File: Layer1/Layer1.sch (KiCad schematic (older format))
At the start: 45 parts, among them IC1 74HCT4060D-Q100,11, J1 Conn_02x20_Odd_Even, J2 Conn_02x20_Odd_Even, J3 Conn_02x12_Odd_Even, J4 Barrel_Jack_MountingPin, SW1 SW_Push, SW2 SW_Push, SW3 SW_DIP_x01, U1 28C256, U10 7400, U11 NE555, U2 74LS193, U3 74461, U4 28C256, U5 74154, U6 74461, U7 28C256, U8 74HCT273, U9 28C256, X1 SG-8002DC

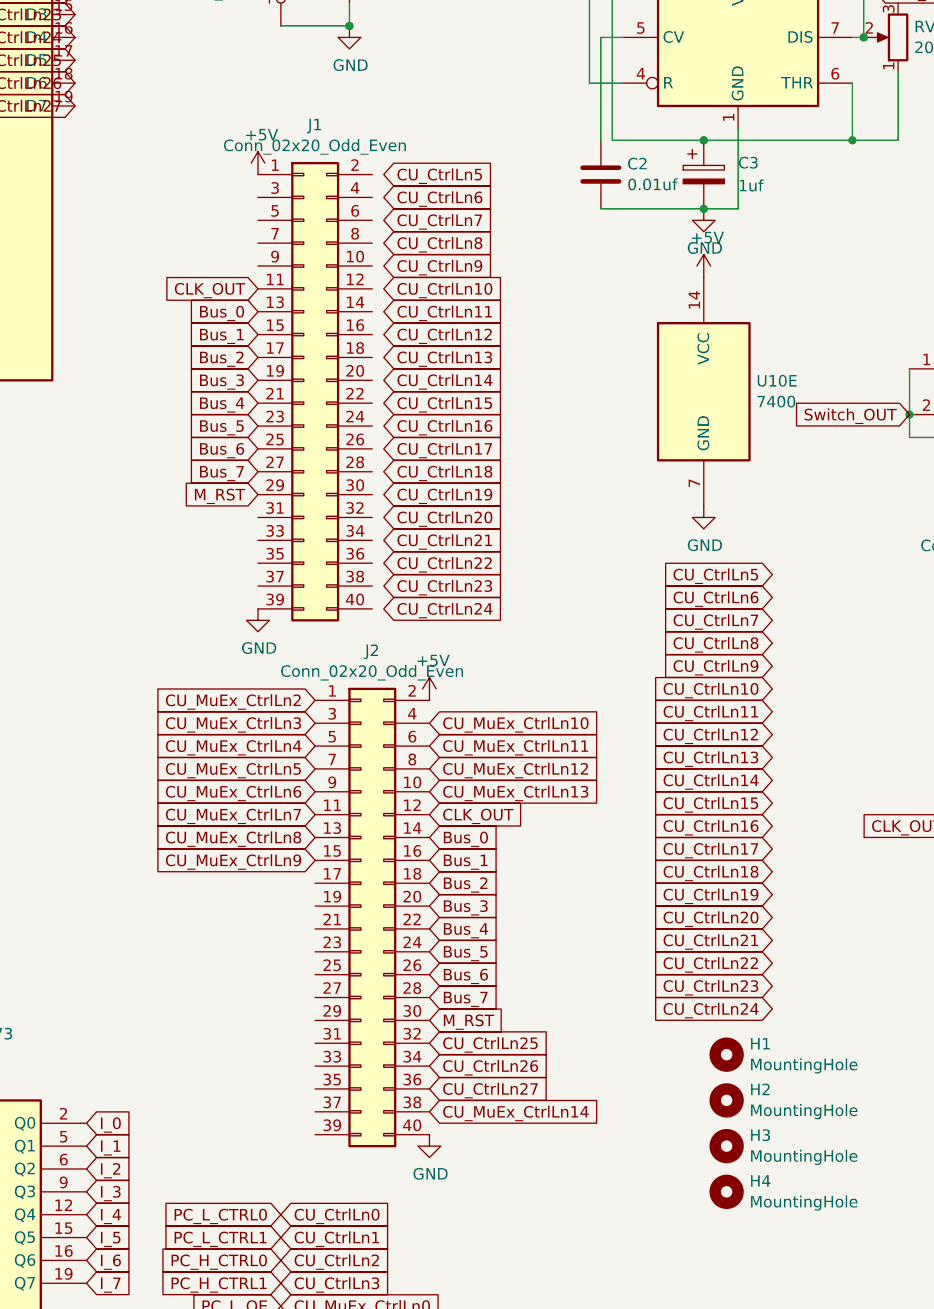
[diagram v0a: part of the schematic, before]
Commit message: Finished Layer1
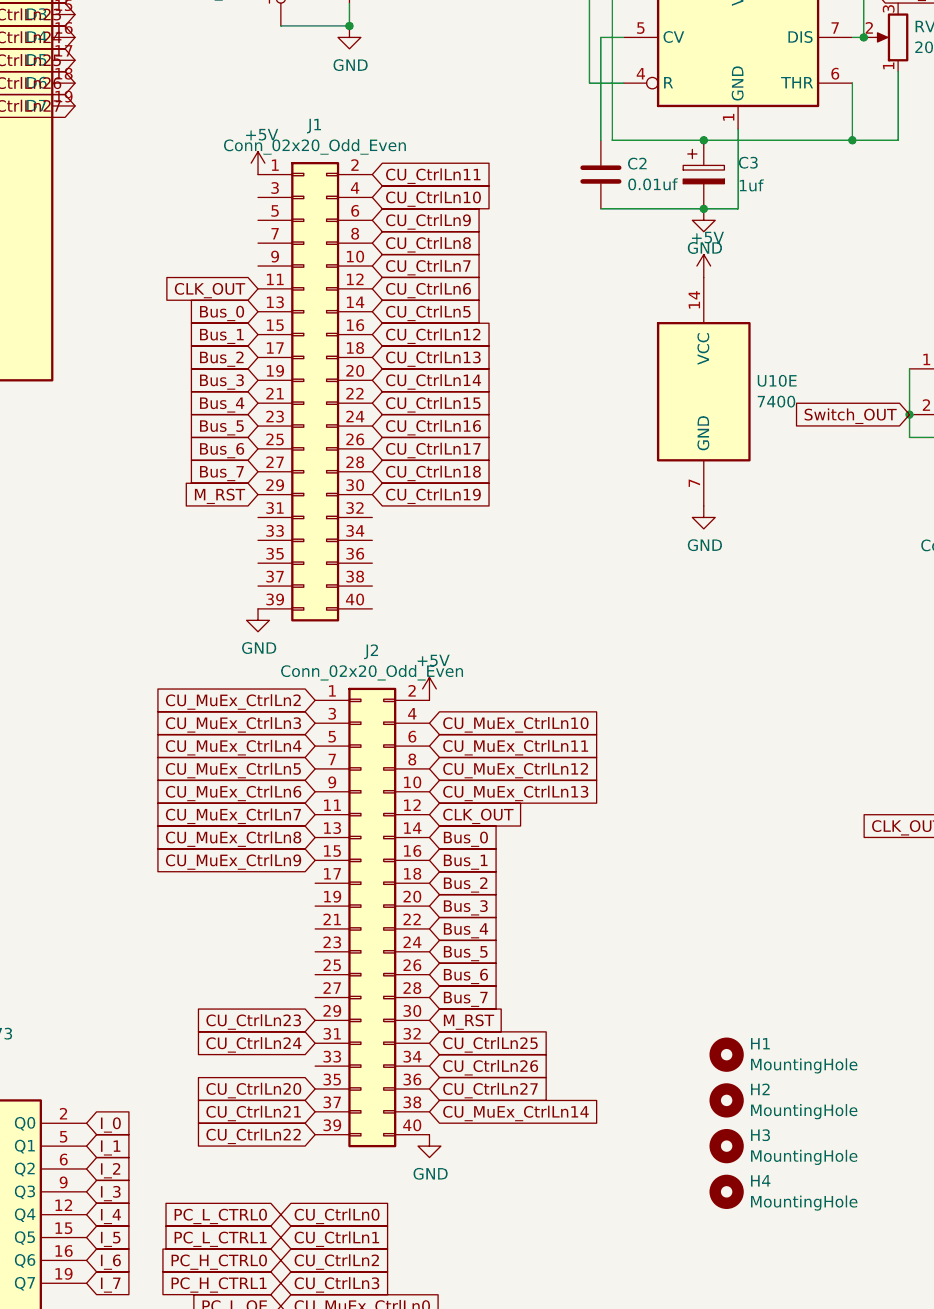
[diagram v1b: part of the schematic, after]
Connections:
- net CU_CtrlLn10: now also J1.4 (Pin_4)
- net CU_CtrlLn11: now also J1.2 (Pin_2)
- net CU_CtrlLn12: now also J1.16 (Pin_16)
- net CU_CtrlLn13: now also J1.18 (Pin_18)
- net CU_CtrlLn14: now also J1.20 (Pin_20)
- net CU_CtrlLn15: now also J1.22 (Pin_22)
- net CU_CtrlLn16: now also J1.24 (Pin_24)
- net CU_CtrlLn17: now also J1.26 (Pin_26)
- net CU_CtrlLn18: now also J1.28 (Pin_28)
- net CU_CtrlLn19: now also J1.30 (Pin_30)
- net CU_CtrlLn20: now also J2.35 (Pin_35)
- net CU_CtrlLn21: now also J2.37 (Pin_37)
- net CU_CtrlLn22: now also J2.39 (Pin_39)
- net CU_CtrlLn23: now also J2.29 (Pin_29)
- net CU_CtrlLn24: now also J2.31 (Pin_31)
- net CU_CtrlLn5: now also J1.14 (Pin_14)
- net CU_CtrlLn6: now also J1.12 (Pin_12)
- net CU_CtrlLn7: now also J1.10 (Pin_10)
- net CU_CtrlLn8: now also J1.8 (Pin_8)
- net CU_CtrlLn9: now also J1.6 (Pin_6)
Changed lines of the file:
@@
 Text GLabel 6600 6050 2    50   Input ~ 0
 CU_MuEx_CtrlLn14
-Text GLabel 6400 1950 2    50   Input ~ 0
-CU_CtrlLn5
-Text GLabel 6400 2050 2    50   Input ~ 0
-CU_CtrlLn6
-Text GLabel 6400 2150 2    50   Input ~ 0
-CU_CtrlLn7
-Text GLabel 6400 2250 2    50   Input ~ 0
-CU_CtrlLn8
-Text GLabel 6400 2350 2    50   Input ~ 0
-CU_CtrlLn9
-Text GLabel 6400 2450 2    50   Input ~ 0
-CU_CtrlLn10
-Text GLabel 6400 2550 2    50   Input ~ 0
-CU_CtrlLn11
-Text GLabel 6400 2650 2    50   Input ~ 0
+Text GLabel 6350 2650 2    50   Input ~ 0
 CU_CtrlLn12
-Text GLabel 6400 2750 2    50   Input ~ 0
+Text GLabel 6350 2750 2    50   Input ~ 0
 CU_CtrlLn13
-Text GLabel 6400 2850 2    50   Input ~ 0
+Text GLabel 6350 2850 2    50   Input ~ 0
 CU_CtrlLn14
-Text GLabel 6400 2950 2    50   Input ~ 0
+Text GLabel 6350 2950 2    50   Input ~ 0
 CU_CtrlLn15
-Text GLabel 6400 3050 2    50   Input ~ 0
+Text GLabel 6350 3050 2    50   Input ~ 0
 CU_CtrlLn16
-Text GLabel 6400 3150 2    50   Input ~ 0
+Text GLabel 6350 3150 2    50   Input ~ 0
 CU_CtrlLn17
-Text GLabel 6400 3250 2    50   Input ~ 0
+Text GLabel 6350 3250 2    50   Input ~ 0
 CU_CtrlLn18
-Text GLabel 6400 3350 2    50   Input ~ 0
+Text GLabel 6350 3350 2    50   Input ~ 0
 CU_CtrlLn19
-Text GLabel 6400 3450 2    50   Input ~ 0
-CU_CtrlLn20
-Text GLabel 6400 3550 2    50   Input ~ 0
-CU_CtrlLn21
-Text GLabel 6400 3650 2    50   Input ~ 0
-CU_CtrlLn22
-Text GLabel 6400 3750 2    50   Input ~ 0
-CU_CtrlLn23
-Text GLabel 6400 3850 2    50   Input ~ 0
-CU_CtrlLn24
 Text GLabel 6600 5750 2    50   Input ~ 0
 CU_CtrlLn25
@@
 Text GLabel 6600 5650 2    50   Input ~ 0
 M_RST
-Text GLabel 8100 3700 0    50   Input ~ 0
+Text GLabel 6100 5950 0    50   Input ~ 0
+CU_CtrlLn20
+Text GLabel 6100 6050 0    50   Input ~ 0
+CU_CtrlLn21
+Text GLabel 6100 6150 0    50   Input ~ 0
+CU_CtrlLn22
+Text GLabel 6100 5650 0    50   Input ~ 0
+CU_CtrlLn23
+Text GLabel 6100 5750 0    50   Input ~ 0
+CU_CtrlLn24
+Text GLabel 6350 1950 2    50   Input ~ 0
+CU_CtrlLn11
+Text GLabel 6350 2050 2    50   Input ~ 0
+CU_CtrlLn10
+Text GLabel 6350 2150 2    50   Input ~ 0
+CU_CtrlLn9
+Text GLabel 6350 2250 2    50   Input ~ 0
+CU_CtrlLn8
+Text GLabel 6350 2350 2    50   Input ~ 0
+CU_CtrlLn7
+Text GLabel 6350 2450 2    50   Input ~ 0
+CU_CtrlLn6
+Text GLabel 6350 2550 2    50   Input ~ 0
 CU_CtrlLn5
-Text GLabel 8100 3800 0    50   Input ~ 0
-CU_CtrlLn6
-Text GLabel 8100 3900 0    50   Input ~ 0
-CU_CtrlLn7
-Text GLabel 8100 4000 0    50   Input ~ 0
-CU_CtrlLn8
-Text GLabel 8100 4100 0    50   Input ~ 0
-CU_CtrlLn9
-Text GLabel 8100 4200 0    50   Input ~ 0
-CU_CtrlLn10
-Text GLabel 8100 4300 0    50   Input ~ 0
-CU_CtrlLn11
-Text GLabel 8100 4400 0    50   Input ~ 0
-CU_CtrlLn12
-Text GLabel 8100 4500 0    50   Input ~ 0
-CU_CtrlLn13
-Text GLabel 8100 4600 0    50   Input ~ 0
-CU_CtrlLn14
-Text GLabel 8100 4700 0    50   Input ~ 0
-CU_CtrlLn15
-Text GLabel 8100 4800 0    50   Input ~ 0
-CU_CtrlLn16
-Text GLabel 8100 4900 0    50   Input ~ 0
-CU_CtrlLn17
-Text GLabel 8100 5000 0    50   Input ~ 0
-CU_CtrlLn18
-Text GLabel 8100 5100 0    50   Input ~ 0
-CU_CtrlLn19
-Text GLabel 8100 5200 0    50   Input ~ 0
-CU_CtrlLn20
-Text GLabel 8100 5300 0    50   Input ~ 0
-CU_CtrlLn21
-Text GLabel 8100 5400 0    50   Input ~ 0
-CU_CtrlLn22
-Text GLabel 8100 5500 0    50   Input ~ 0
-CU_CtrlLn23
-Text GLabel 8100 5600 0    50   Input ~ 0
-CU_CtrlLn24
 $EndSCHEMATC
